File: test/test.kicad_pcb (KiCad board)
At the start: 2 copper layers, 25.4 x 25.4 mm, 3 parts, among them U1 AP2112K-3.3, U2 ATmega32U4-AU

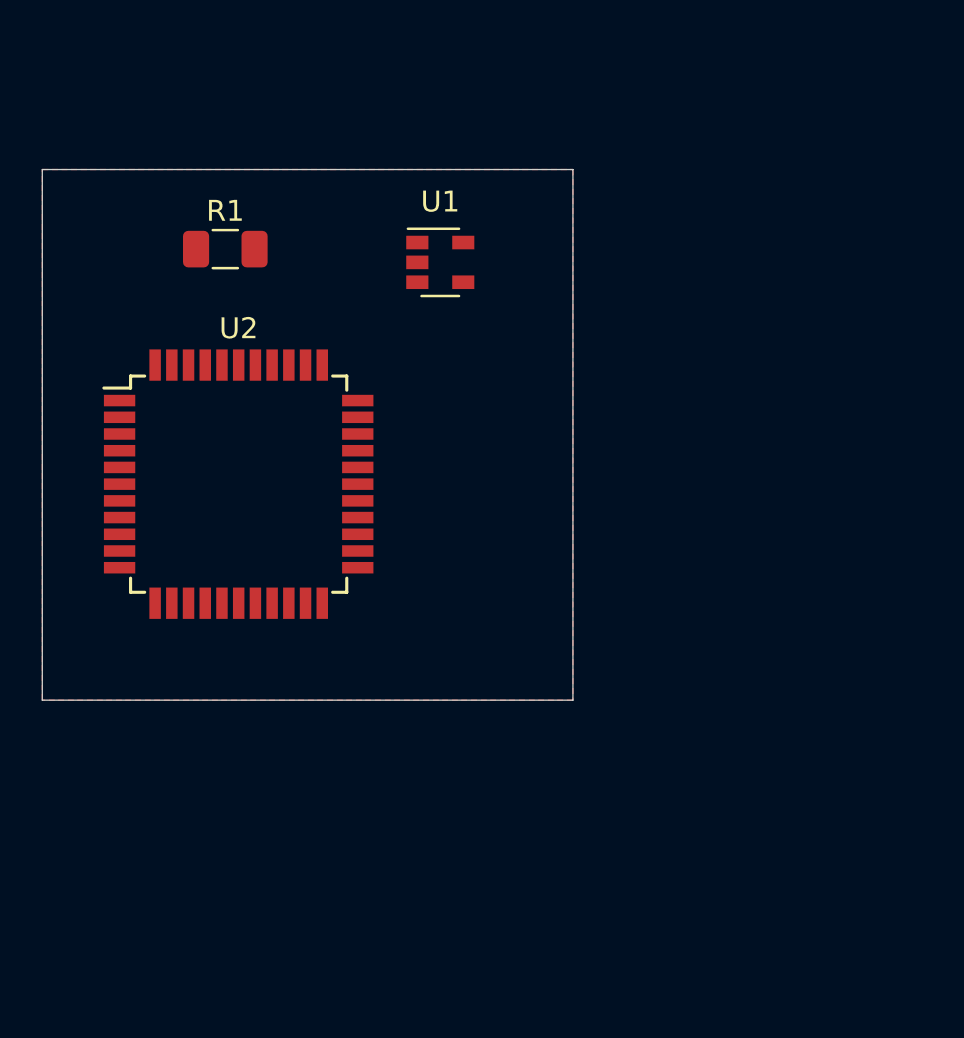
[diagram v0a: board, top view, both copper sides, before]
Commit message: update
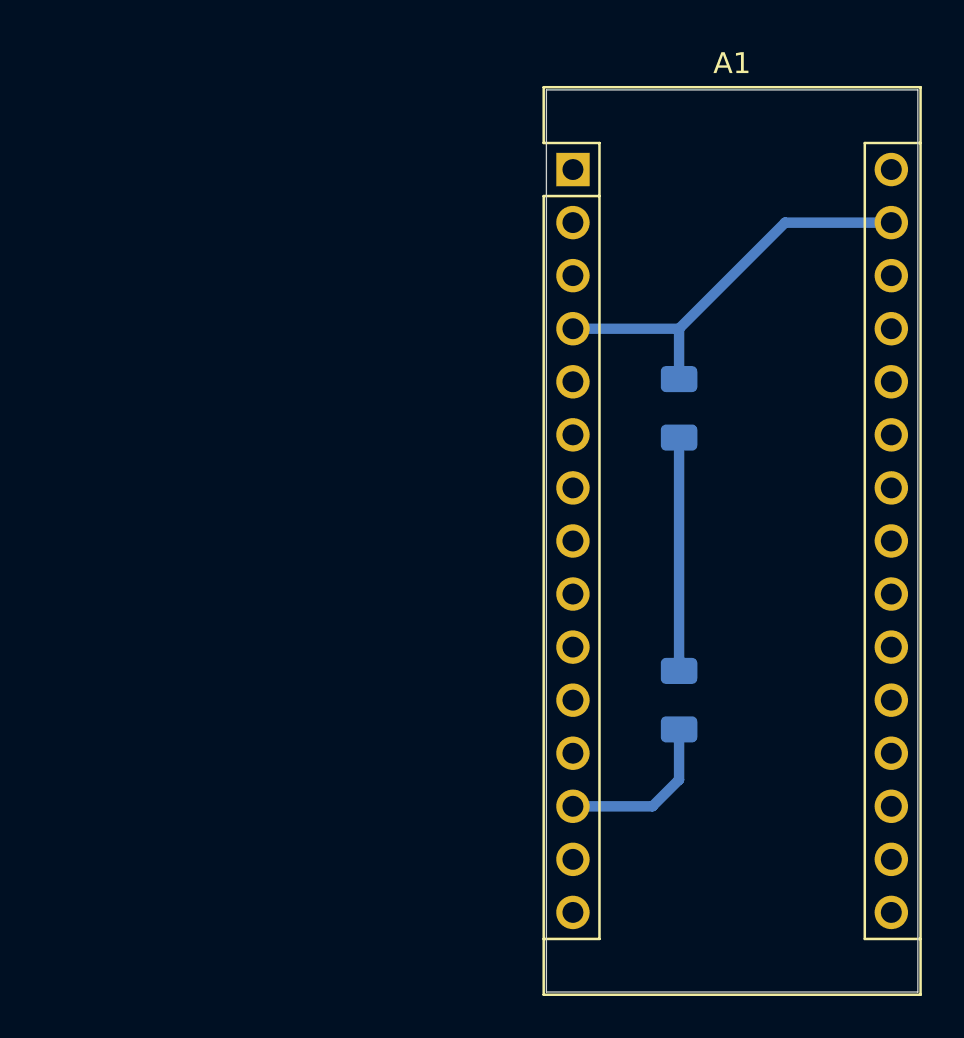
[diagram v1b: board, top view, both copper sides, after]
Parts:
- removed U1: AP2112K-3.3, Package_TO_SOT_SMD:SOT-23-5
- removed U2: ATmega32U4-AU, Package_QFP:TQFP-44_10x10mm_P0.8mm
- added A1: Arduino_Nano_v2.x, Module:Arduino_Nano, F.Cu at (127.0, 76.2)
- added D1: LED, LED_SMD:LED_1206_3216Metric, B.Cu at (132.1, 101.6)
- R1: moved to B.Cu
- moved R1 23.0 mm to (132.1, 87.6), turned to 90 degrees
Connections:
- R1 pad 1: (no net) -> Net-(D1-Pad1)
- R1 pad 2: Net-(R1-Pad2) -> GND
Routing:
- net GND: track 0.00 -> 19.8 mm
- net Net-(D1-Pad1): track 0.00 -> 11.2 mm
- net Net-(A1-Pad13): track 0.00 -> 8.02 mm
- removed copper zone on F.Cu, net Net-(R1-Pad2)
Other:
- board size 25.4 x 25.4 mm -> 17.8 x 43.2 mm
